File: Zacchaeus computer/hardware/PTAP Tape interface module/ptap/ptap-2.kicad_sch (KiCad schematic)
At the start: 45 parts, among them J2 Conn_01x02_Pin, J3 Conn_01x02_Pin, J4 Conn_01x02_Pin, J5 Conn_01x02_Pin, J6 Conn_01x02_Pin, K1 LEG-5, Q1 2N2219, Q2 BC548C, Q3 BC548C, Q4 BC548C, Q5 BC548C, Q6 BC548C, Q7 BC548C, Q8 BC548C, U4 74LS373, U5 74LS245, U6 DS87C520, Y1 11.0592 MHz

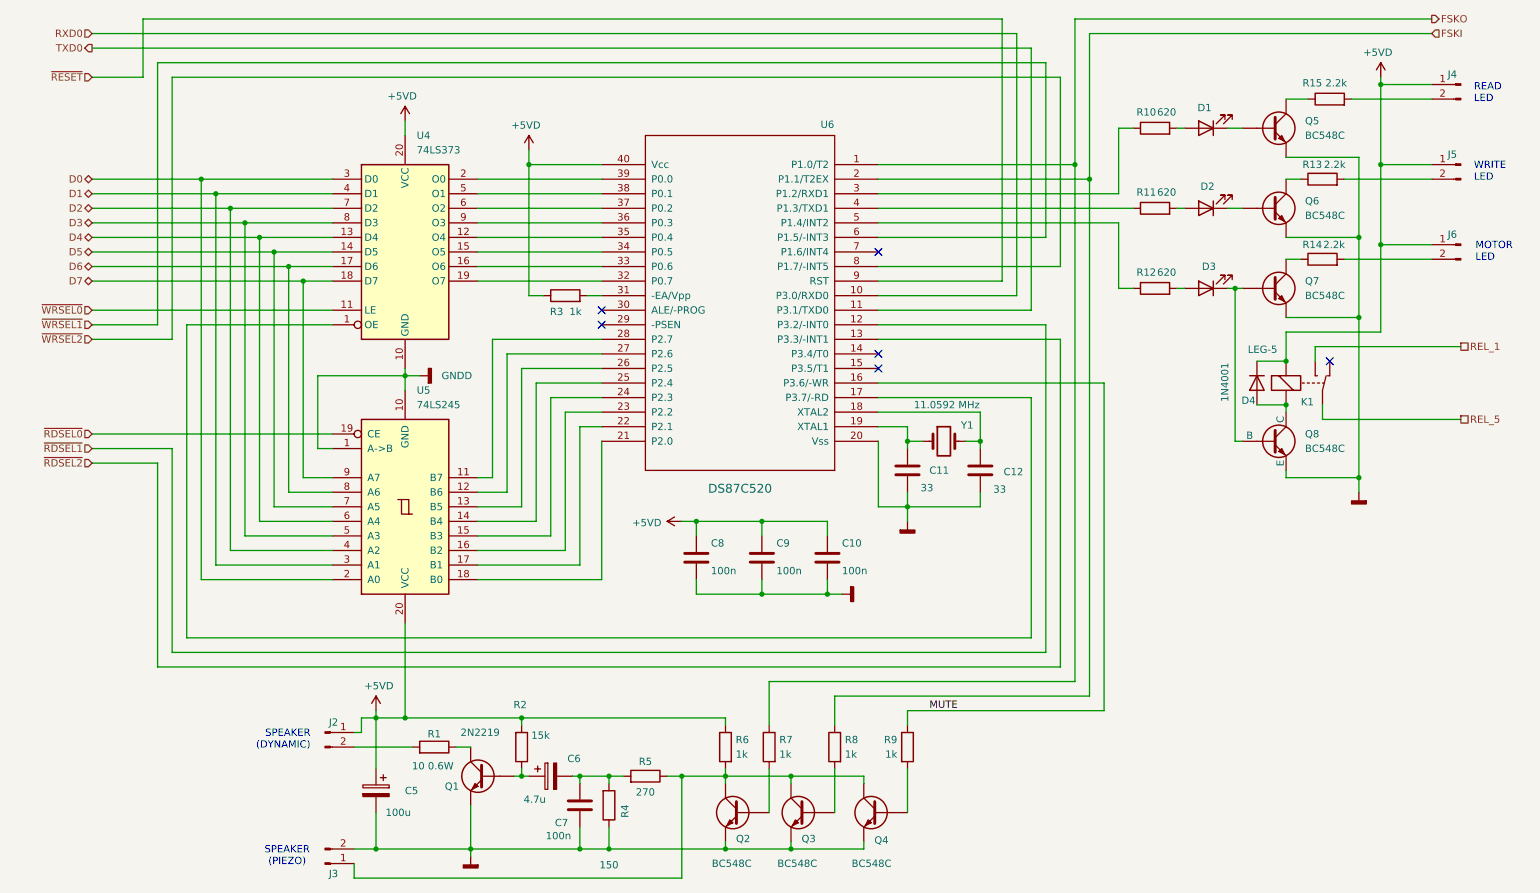
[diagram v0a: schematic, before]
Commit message: 260405
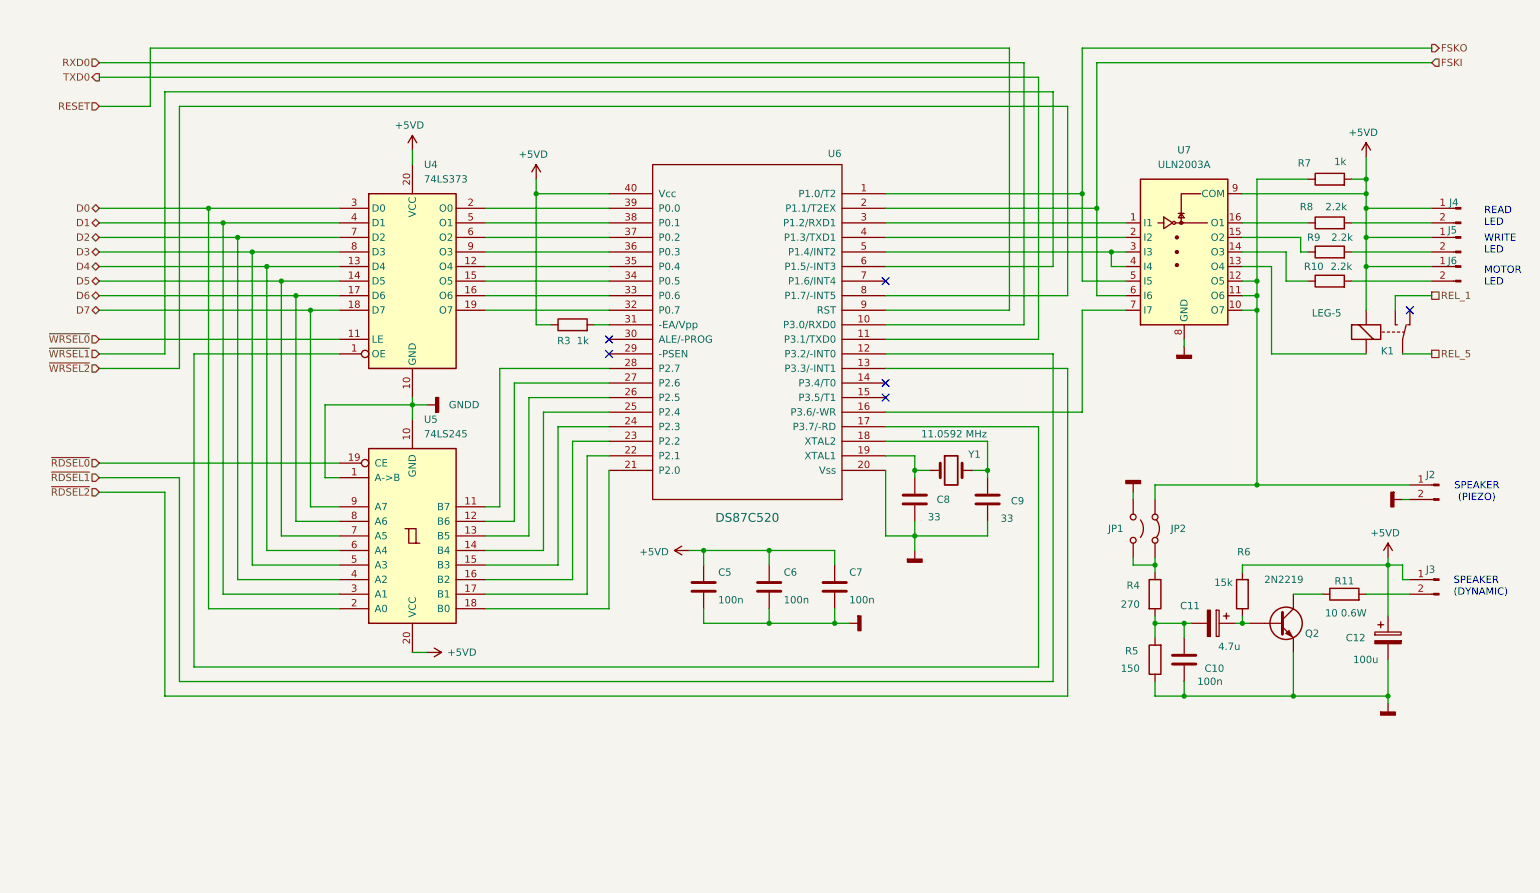
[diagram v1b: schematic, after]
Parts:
- removed D1, D2, D3: LED, symbol Device:LED
- removed D4: 1N4001, symbol Device:D
- removed Q2, Q3, Q4, Q5, Q6, Q7, Q8: BC548C, symbol Simulation_SPICE:NPN
- removed R10, R11, R12: 620, symbol Device:R
- removed R7, R8, R9: 1k, symbol Device:R
- added JP1: Jumper_2_Open, symbol Jumper:Jumper_2_Open
- added JP2: Jumper_2_Bridged, symbol Jumper:Jumper_2_Bridged
- added U7: ULN2003A, symbol Transistor_Array:ULN2003A
- renumbered C7 to C10, C6 to C11, C5 to C12, C8 to C5, C9 to C6, C10 to C7, C11 to C8, C12 to C9, J3 to J2, J2 to J3, Q1 to Q2, R14 to R10, R1 to R11, R5 to R4, R4 to R5, R2 to R6, R6 to R7, R15 to R8, R13 to R9
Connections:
- net +5VD: now also R7.2, U7.9 (COM); no longer R7.1
- net FSKI: now also U7.6 (I6)
- net FSKO: now also U7.5 (I5)
- net GNDD: now also JP1.2 (B), U7.8 (GND)
- net at R8.1: now also U7.16 (O1)
- net at R10.1: now also U7.14 (O3)
- net at U6.4 (P1.3/TXD1): now also U7.2 (I2)
- net at K1.2 (Coil): now also U7.13 (O4)
- net at U6.5 (P1.4/INT2): now also U7.3 (I3), U7.4 (I4)
- net at U6.3 (P1.2/RXD1): now also U7.1 (I1)
- net at R9.1: now also U7.15 (O2)
- net MUTE: no longer names the net of U6.16 (P3.6/-WR)
- net MUTE: now also U7.7 (I7)
- net ~{RESET} renamed RESET
- new net: J2.1 (Pin_1), JP2.2 (B), R7.1, U7.10 (O7), U7.11 (O6), U7.12 (O5)
- new net: JP1.1 (A), JP2.1 (A), R4.1
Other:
- moved on the sheet: C10, C11, C12, C5, C6, C7, C8, C9, J2, J3, J4, J5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
